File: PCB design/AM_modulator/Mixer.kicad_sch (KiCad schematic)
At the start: 7 parts

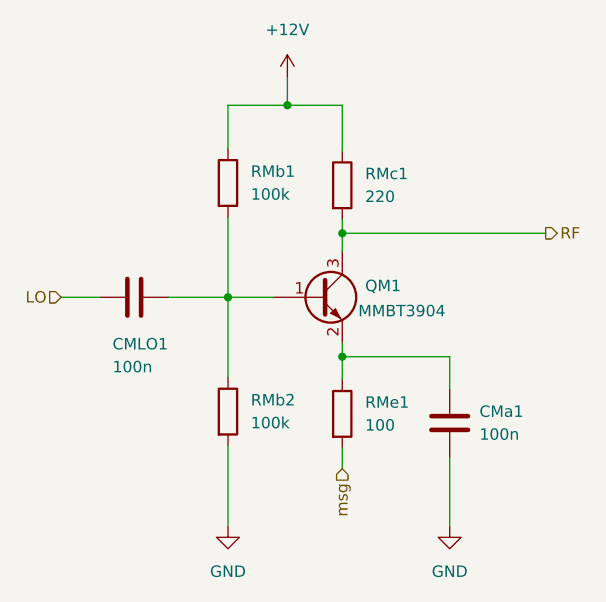
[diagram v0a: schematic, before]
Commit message: PCB design done
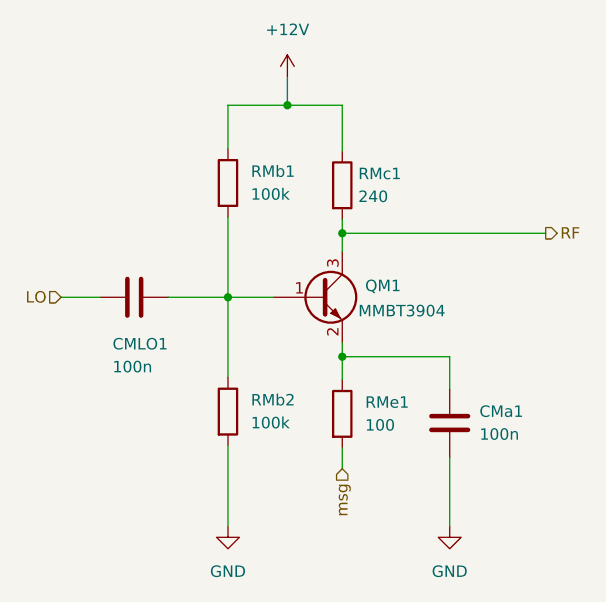
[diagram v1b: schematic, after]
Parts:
- RMc1: value 220 -> 240; footprint Resistor_SMD:R_0805_2012Metric_Pad1.20x1.40mm_HandSolder -> Resistor_SMD:R_1206_3216Metric_Pad1.30x1.75mm_HandSolder
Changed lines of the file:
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@@
   (symbol (lib_id "Device:R") (at 139.192 76.454 0) (unit 1)
     (in_bom yes) (on_board yes) (fields_autoplaced)
-    (property "Reference" "RMc1" (id 0) (at 141.732 75.1839 0)
+    (property "Reference" "RMc1" (id 0) (at 140.97 75.1839 0)
       (effects (font (size 1.27 1.27)) (justify left))
     )
-    (property "Value" "220" (id 1) (at 141.732 77.7239 0)
+    (property "Value" "240" (id 1) (at 140.97 77.7239 0)
       (effects (font (size 1.27 1.27)) (justify left))
     )
-    (property "Footprint" "Resistor_SMD:R_0805_2012Metric_Pad1.20x1.40mm_HandSolder" (id 2) (at 137.414 76.454 90)
+    (property "Footprint" "Resistor_SMD:R_1206_3216Metric_Pad1.30x1.75mm_HandSolder" (id 2) (at 137.414 76.454 90)
       (effects (font (size 1.27 1.27)) hide)
     )
